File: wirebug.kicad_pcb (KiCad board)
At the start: 2 copper layers, 53.3 x 50.8 mm, 5 parts

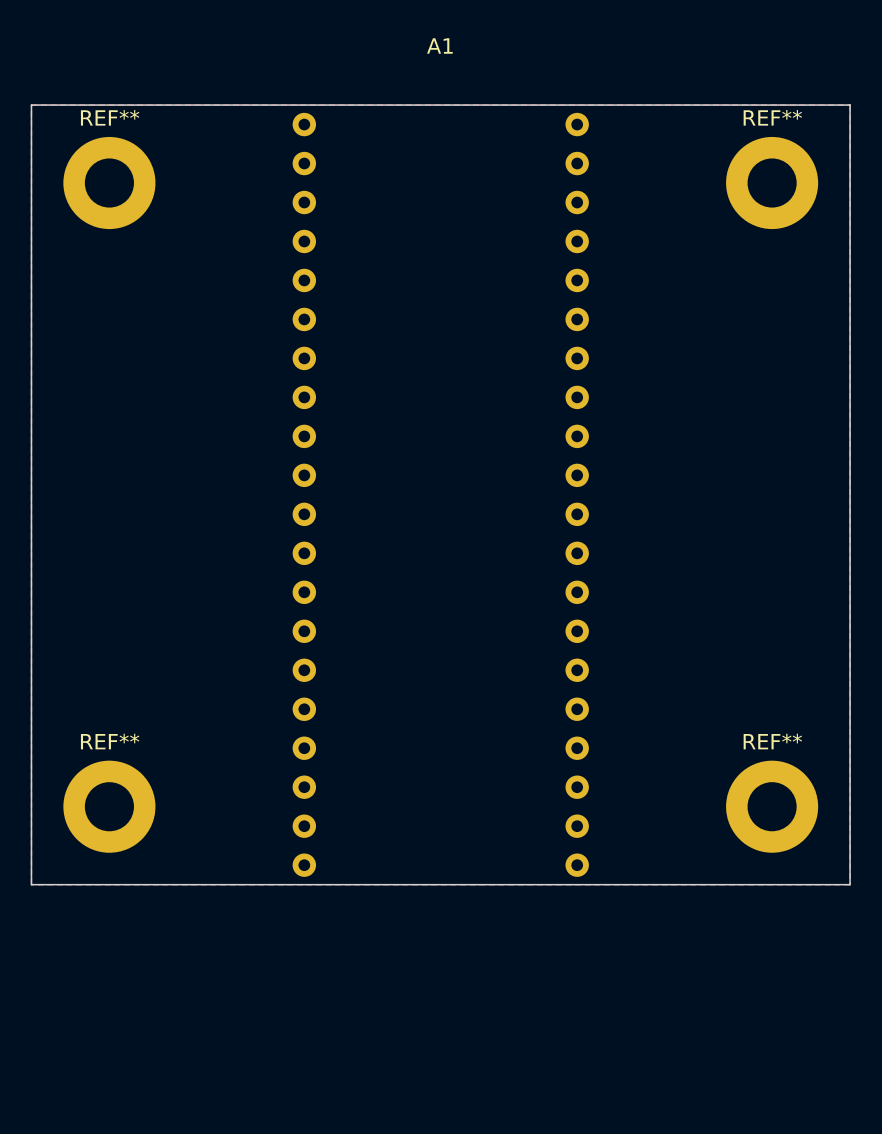
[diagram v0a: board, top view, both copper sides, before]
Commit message: First draft
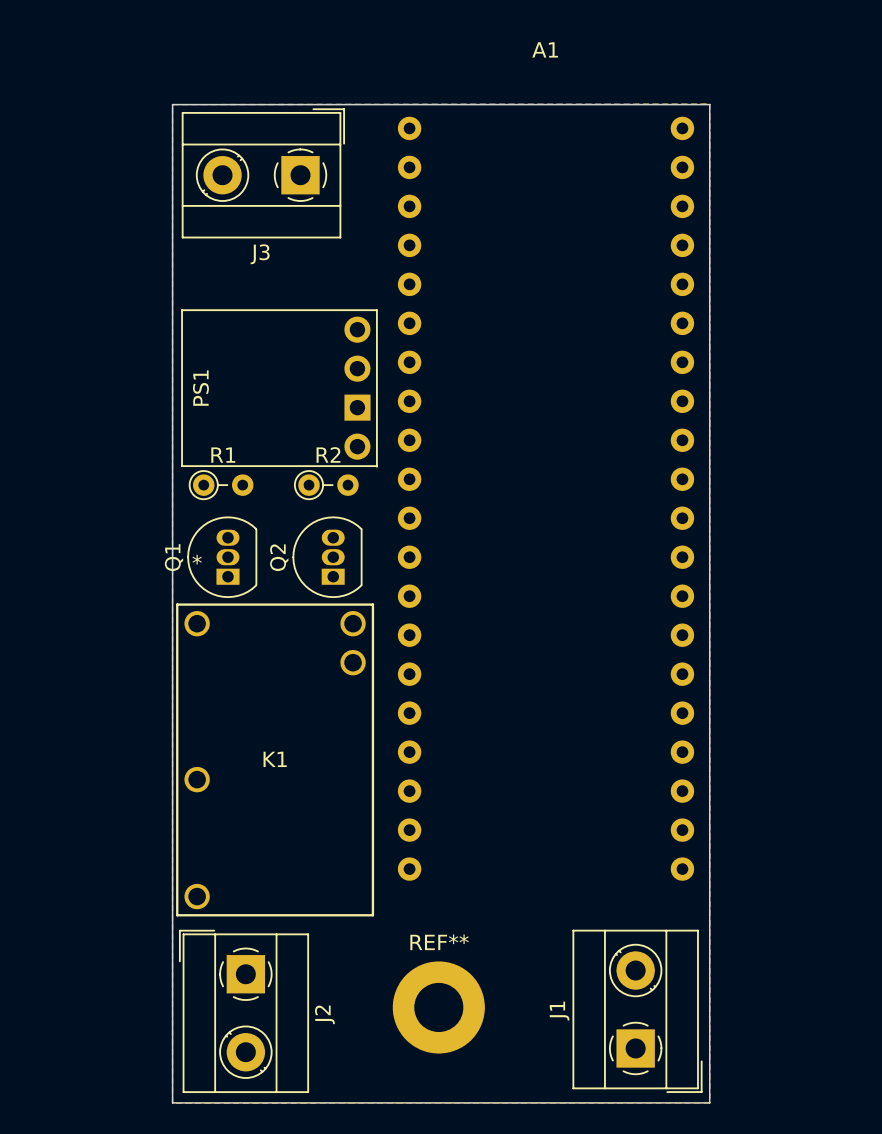
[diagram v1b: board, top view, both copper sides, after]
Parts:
- removed the REF** at (147.3, 96.5)
- removed the REF** at (104.1, 55.9)
- removed the REF** at (147.3, 55.9)
- added J1: Screw_Terminal_01x02, twyleg-connectors:TerminalBlock_MetzConnect_Type101_RT01602HBWC_1x02_P5.08mm_Horizontal, F.Cu at (138.4, 112.3)
- added J2: Screw_Terminal_01x02, twyleg-connectors:TerminalBlock_MetzConnect_Type101_RT01602HBWC_1x02_P5.08mm_Horizontal, F.Cu at (113.0, 107.4)
- added J3: Screw_Terminal_01x02, twyleg-connectors:TerminalBlock_MetzConnect_Type101_RT01602HBWC_1x02_P5.08mm_Horizontal, F.Cu at (116.6, 55.4)
- added K1: AW3211F, twyleg-misc:Relay_Panasonic_AW3211F_THT, F.Cu at (109.9, 84.6)
- added PS1: Pololu-D24V5F3, twyleg-voltage-regulators:Pololu-D24V5F3-Dev, F.Cu at (121.6, 74.3)
- added Q1: BC337, Package_TO_SOT_THT:TO-92_Inline, F.Cu at (111.9, 81.5)
- added Q2: BC337, Package_TO_SOT_THT:TO-92_Inline, F.Cu at (118.7, 81.5)
- added R1: 1K, Resistor_THT:R_Axial_DIN0204_L3.6mm_D1.6mm_P2.54mm_Vertical, F.Cu at (110.3, 75.6)
- added R2: 1K, Resistor_THT:R_Axial_DIN0204_L3.6mm_D1.6mm_P2.54mm_Vertical, F.Cu at (117.1, 75.6)
- moved REF** 25.1 mm to (125.6, 109.6)
- moved A1 6.86 mm to (132.6, 52.3)
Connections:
- A1 pad 19: unconnected-(A1-GP14|SPI1_SCK|I2C1_SDA-Pad19) -> /SET
- A1 pad 20: unconnected-(A1-GP15|SPI1_TXD|I2C1_SCL-Pad20) -> /RESET
- A1 pad 36: unconnected-(A1-3V3(OUT)-Pad36) -> /3V3
- A1 pad 38: unconnected-(A1-GND-Pad38) -> /GND
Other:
- board size 53.3 x 50.8 mm -> 35 x 65 mm
